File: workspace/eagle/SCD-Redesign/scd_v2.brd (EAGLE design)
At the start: 77.8 x 45.7 mm, 21 parts, among them J1 AVR_SPI_PRG_6PTH, U2 ATMEGA328P_TQFP

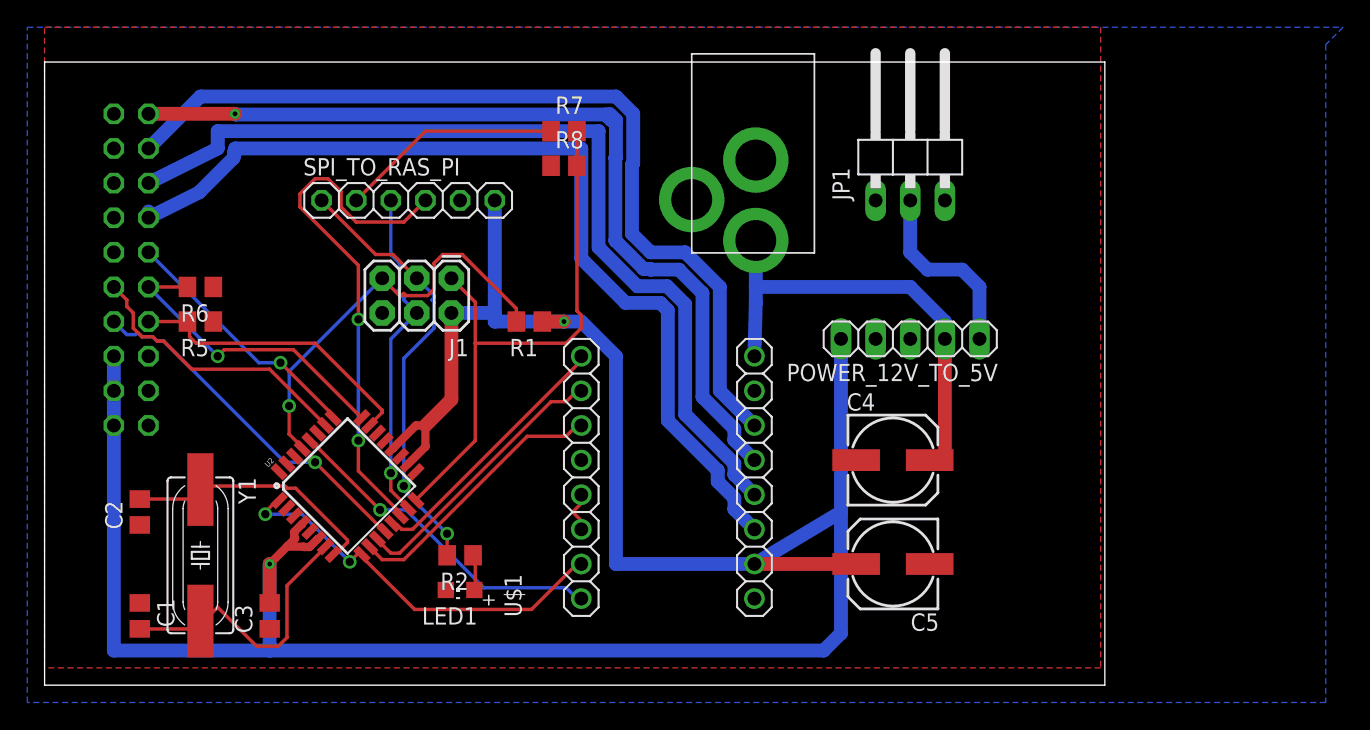
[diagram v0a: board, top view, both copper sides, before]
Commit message: eagle files uploaded
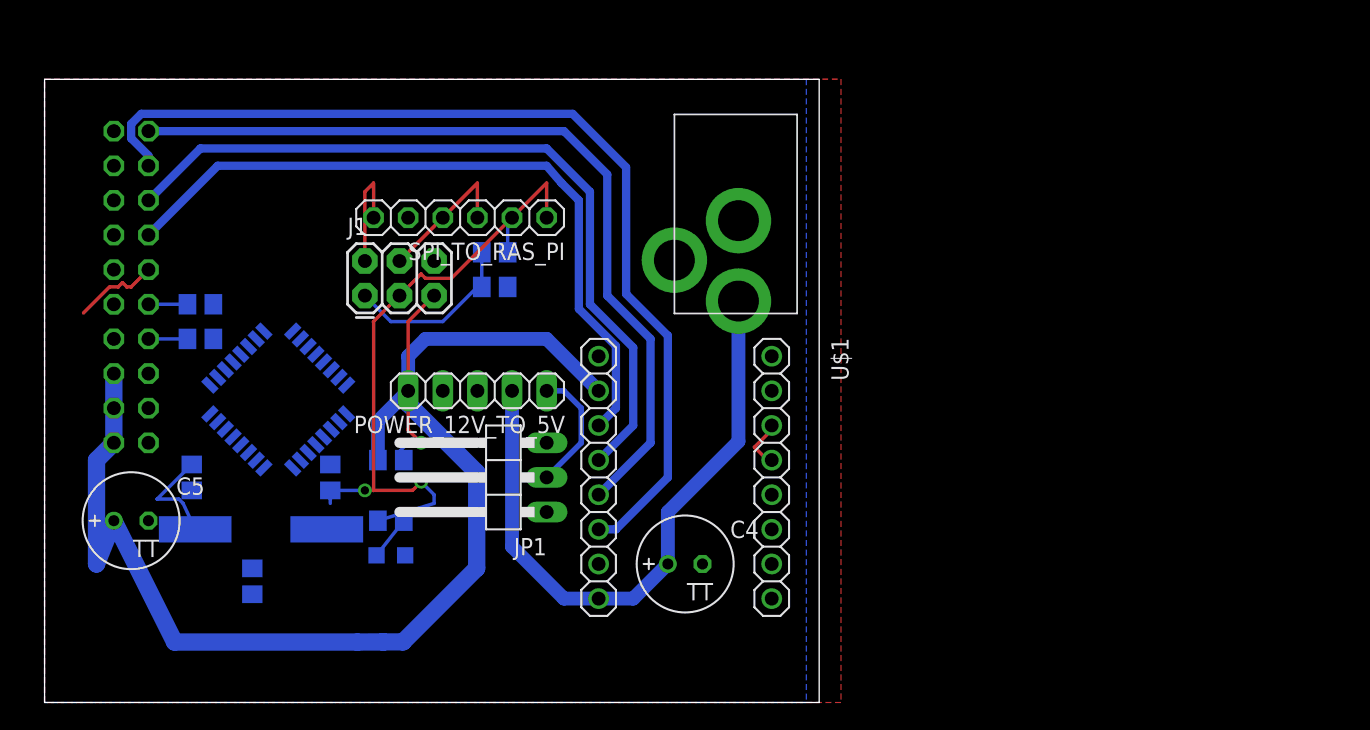
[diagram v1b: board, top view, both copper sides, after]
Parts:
- C4, C5: device rcl:153CLV-0605 -> resistor:TT2D7
- moved C5 56.0 mm to (6.35, 19.7), turned to 0 degrees
- moved JP1 38.9 mm to (33.0, 22.9), turned to 90 degrees
- moved POWER_12V_TO_5V 32.0 mm to (31.8, 29.2)
- moved U$1 23.3 mm to (52.1, 33.0), turned to 270 degrees
- moved C1 17.3 mm to (21.0, 22.9), flipped to the bottom, turned to 90 degrees
- moved C4 17.0 mm to (47.0, 16.5)
- moved R1 14.4 mm to (25.4, 24.1), flipped to the bottom
- moved R7 10.2 mm to (33.0, 39.4), flipped to the bottom
- moved R8 10.2 mm to (33.0, 36.8), flipped to the bottom
- moved U2 8.13 mm to (17.1, 28.6), flipped to the bottom, turned to 135 degrees
- moved J1 6.48 mm to (23.5, 36.2), turned to 0 degrees
- moved LED1 5.68 mm to (25.4, 17.1), flipped to the bottom
- moved R2 5.68 mm to (25.4, 19.7), flipped to the bottom, turned to 0 degrees
- moved Y1 4.84 mm to (15.9, 19.1), flipped to the bottom, turned to 180 degrees
- moved POWER_12V 4.62 mm to (50.8, 45.1)
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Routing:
- net 5V: track 193.0 -> 100.6 mm, vias 2 -> 0
- net SS: track 39.0 -> 0.00 mm, vias 2 -> 0
- net N$5: track 29.6 -> 0.32 mm, vias 2 -> 0
- net MISO: track 41.6 -> 13.1 mm
- net N$13: track 26.4 -> 0.00 mm, vias 1 -> 0
- net N$14: track 24.7 -> 0.00 mm, vias 1 -> 0
- net N$8: track 21.0 -> 0.00 mm
- net N$19: track 20.7 -> 0.00 mm
- net MS1: track 20.7 -> 0.00 mm
- net N$17: track 22.9 -> 2.86 mm, vias 1 -> 0
- net N$12: track 19.8 -> 0.00 mm
- net MS2: track 20.0 -> 0.32 mm
- net N$16: track 22.0 -> 2.86 mm
- net RESET: track 31.2 -> 15.0 mm
- net N$20: track 69.0 -> 52.9 mm
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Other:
- board size 77.8 x 45.7 mm -> 56.8 x 45.7 mm
